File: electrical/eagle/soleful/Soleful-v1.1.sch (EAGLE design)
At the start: 118 parts, among them CN1 To Battery, CN2 Ext Power, IC1 STM32F405RGT, IC2 LT1129-3.3, IC3 MCP73833-UN, Q4 32.768kHz, SW1 RST, U1 USB Power, U2 TPD3E001DRLR, Y1 12 MHz, Y2 32.768kHz

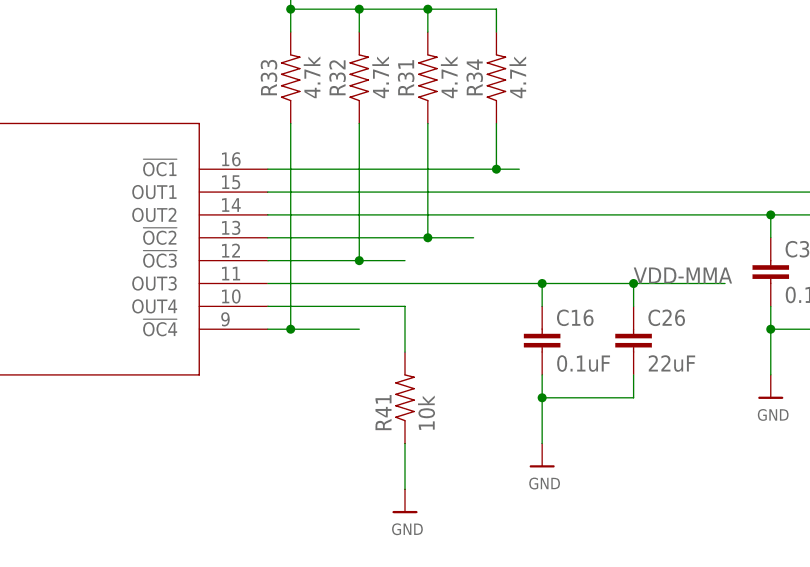
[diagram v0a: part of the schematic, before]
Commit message: finished board layout bitch
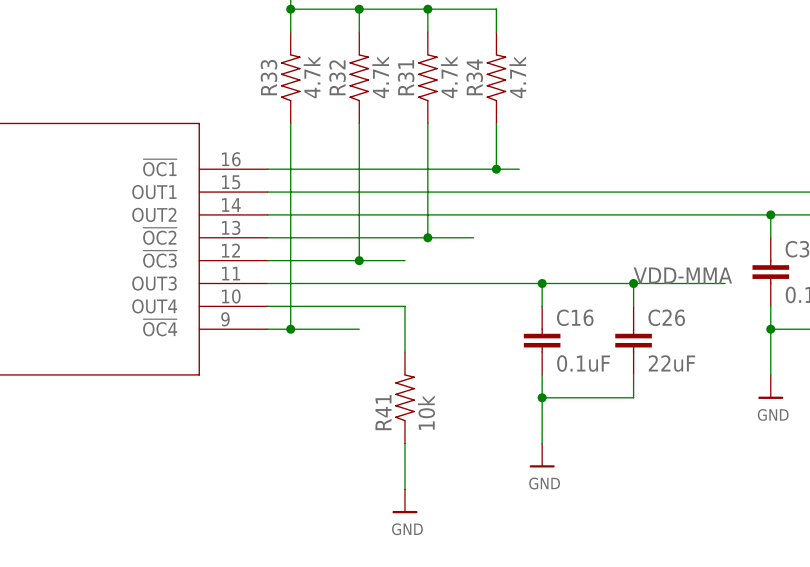
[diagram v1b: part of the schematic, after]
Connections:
- removed net N$19: U$18.OUT4
- removed net N$23: R41.2
- net N$16: now also R41.2, U$18.OUT4; no longer U$18.OUT3
- net VDD-MMA: now also U$18.OUT3
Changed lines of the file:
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@@
-</segment>
-</net>
-<net name="N$16" class="0">
-<segment>
-<pinref part="U$18" gate="A" pin="OUT3"/>
-<wire x1="332.74" y1="121.92" x2="358.14" y2="121.92" width="0.1524" layer="91"/>
-</segment>
-</net>
-<net name="N$19" class="0">
-<segment>
-<pinref part="U$18" gate="A" pin="OUT4"/>
-<wire x1="332.74" y1="119.38" x2="347.98" y2="119.38" width="0.1524" layer="91"/>
 </segment>
 </net>
@@
 <net name="VDD-MMA" class="0">
 <segment>
-<wire x1="358.14" y1="121.92" x2="363.22" y2="121.92" width="0.1524" layer="91"/>
 <wire x1="363.22" y1="121.92" x2="363.22" y2="119.38" width="0.1524" layer="91"/>
 <wire x1="363.22" y1="121.92" x2="373.38" y2="121.92" width="0.1524" layer="91"/>
-<junction x="363.22" y="121.92"/>
 <wire x1="373.38" y1="121.92" x2="373.38" y2="119.38" width="0.1524" layer="91"/>
 <wire x1="373.38" y1="121.92" x2="383.54" y2="121.92" width="0.1524" layer="91"/>
@@
 <pinref part="C26" gate="G$1" pin="1"/>
 <label x="373.38" y="121.92" size="1.778" layer="95"/>
+<pinref part="U$18" gate="A" pin="OUT3"/>
+<wire x1="332.74" y1="121.92" x2="363.22" y2="121.92" width="0.1524" layer="91"/>
+<junction x="363.22" y="121.92"/>
 </segment>
 <segment>
@@
 </segment>
 </net>
-<net name="N$23" class="0">
-<segment>
-<wire x1="347.98" y1="119.38" x2="347.98" y2="114.3" width="0.1524" layer="91"/>
-<pinref part="R41" gate="G$1" pin="2"/>
-</segment>
-</net>
 <net name="N$26" class="0">
 <segment>
@@
 </segment>
 </net>
+<net name="N$16" class="0">
+<segment>
+<pinref part="U$18" gate="A" pin="OUT4"/>
+<pinref part="R41" gate="G$1" pin="2"/>
+<wire x1="332.74" y1="119.38" x2="347.98" y2="119.38" width="0.1524" layer="91"/>
+<wire x1="347.98" y1="119.38" x2="347.98" y2="114.3" width="0.1524" layer="91"/>
+</segment>
+</net>
